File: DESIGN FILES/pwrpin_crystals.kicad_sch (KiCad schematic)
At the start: 34 parts, among them U1 MIMXRT1064CVL5B, Y1 7V24000026, Y2 X201232768KJD2SI

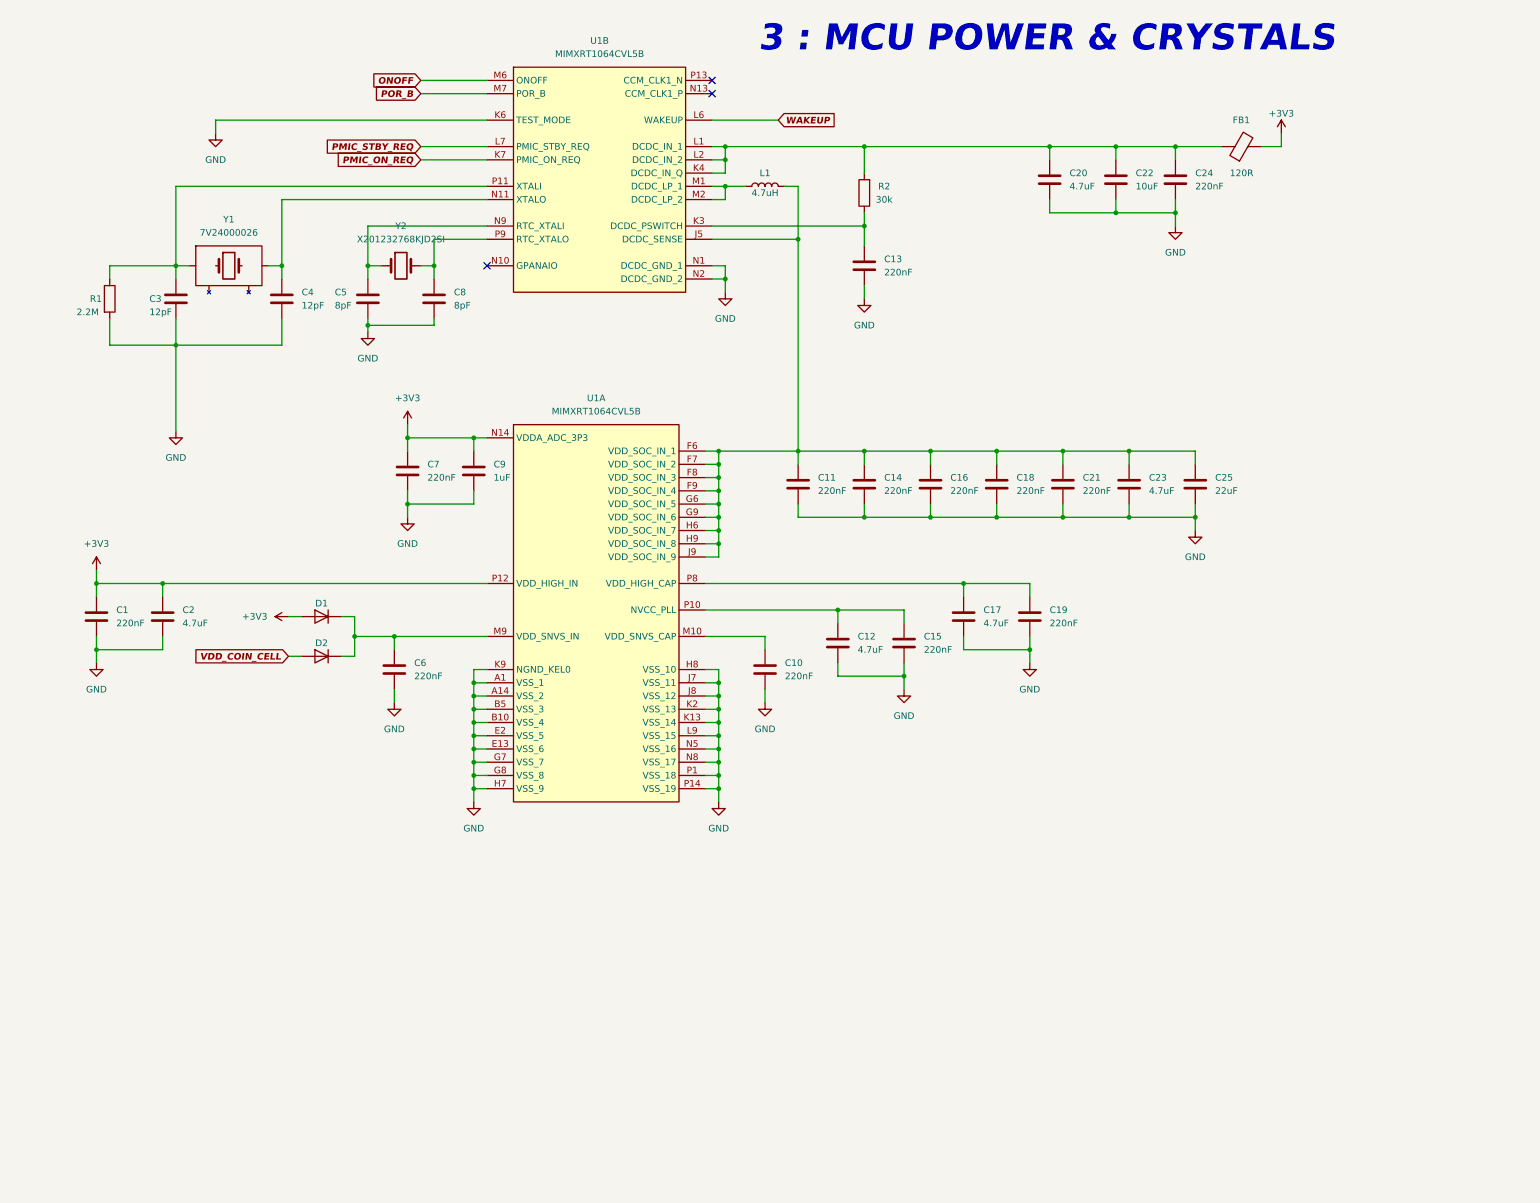
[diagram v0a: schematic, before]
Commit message: schematic edit
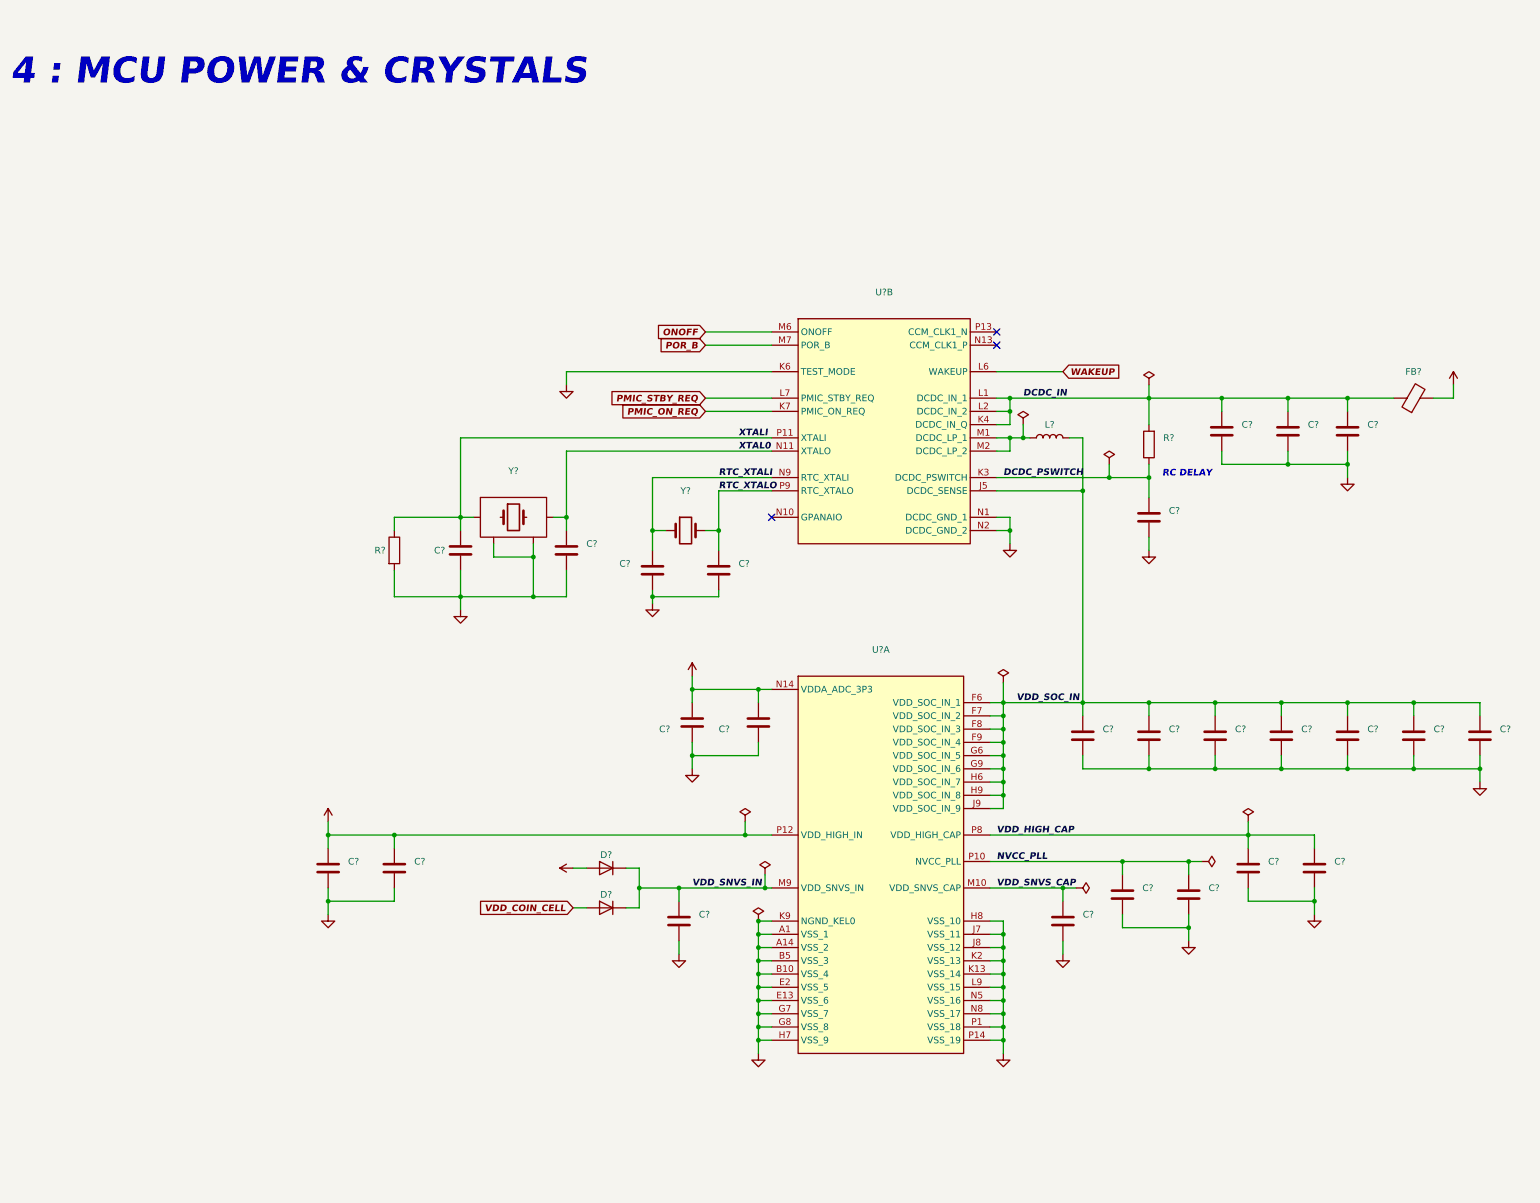
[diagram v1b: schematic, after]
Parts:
- removed C1, C10, C11, C13, C14, C15, C16, C18, C19, C21, C24, C6, C7: 220nF, MIMXRT1064 MCU Module:0402_CL05B224KO5NNNC, symbol MIMXRT1064 MCU Module:CL05B224KO5NNNC
- removed C12, C17, C2, C20, C23: 4.7uF, MIMXRT1064 MCU Module:0402_CL05A475MP5NRNC, symbol MIMXRT1064 MCU Module:CL05A475MP5NRNC
- removed C22: 10uF, MIMXRT1064 MCU Module:0603_CL10A106KP8NNNC, symbol MIMXRT1064 MCU Module:CL10A106KP8NNNC
- removed C25: 22uF, MIMXRT1064 MCU Module:0603_CL10A226MQ8NRNC, symbol MIMXRT1064 MCU Module:CL10A226MQ8NRNC
- removed C3, C4: 12pF, MIMXRT1064 MCU Module:0402_GRM1555C1H120GA01D, symbol MIMXRT1064 MCU Module:GRM1555C1H120GA01D
- removed C5, C8: 8pF, MIMXRT1064 MCU Module:0402_GCM1555C1H8R0DA16D, symbol MIMXRT1064 MCU Module:GCM1555C1H8R0DA16D
- removed C9: 1uF, MIMXRT1064 MCU Module:0402_CL05A105KA5NQNC, symbol MIMXRT1064 MCU Module:CL05A105KA5NQNC
- removed D1, D2: RB521S30_R1_00001, MIMXRT1064 MCU Module:RB521S30_R1_00001, symbol MIMXRT1064 MCU Module:RB521S30_R1_00001
- removed FB1: 120R, MIMXRT1064 MCU Module:0603_BLM18AG121SN1D, symbol MIMXRT1064 MCU Module:BLM18AG121SN1D
- removed L1: 4.7uH, MIMXRT1064 MCU Module:CD32YP0302-4R7M, symbol MIMXRT1064 MCU Module:CD32YP0302-4R7M
- removed R1: 2.2M, MIMXRT1064 MCU Module:0402WGJ0225TCE, symbol MIMXRT1064 MCU Module:0402WGJ0225TCE
- removed R2: 30k, MIMXRT1064 MCU Module:TC0225F3002TCE, symbol MIMXRT1064 MCU Module:TC0225F3002TCE
- removed U1: MIMXRT1064CVL5B, MIMXRT1064 MCU Module:MIMXRT1064CVL5B, symbol MIMXRT1064 MCU Module:MIMXRT1064CVL5B
- removed Y1: 7V24000026, MIMXRT1064 MCU Module:7V24000026, symbol MIMXRT1064 MCU Module:7V24000026
- removed Y2: X201232768KJD2SI, MIMXRT1064 MCU Module:X201232768KJD2SI, symbol MIMXRT1064 MCU Module:X201232768KJD2SI
- added C? (x13): ~, symbol MIMXRT1064 MCU Module:CL05B224KO5NNNC
- added C?: ~, symbol MIMXRT1064 MCU Module:CL10A106KP8NNNC
- added C? (x2): ~, symbol MIMXRT1064 MCU Module:GCM1555C1H8R0DA16D
- added C?: ~, symbol MIMXRT1064 MCU Module:CL05A105KA5NQNC
- added C? (x5): ~, symbol MIMXRT1064 MCU Module:CL05A475MP5NRNC
- added C?: ~, symbol MIMXRT1064 MCU Module:CL10A226MQ8NRNC
- added C? (x2): ~, symbol MIMXRT1064 MCU Module:GRM1555C1H120GA01D
- added D? (x2): ~, symbol MIMXRT1064 MCU Module:RB521S30_R1_00001
- added FB?: ~, symbol MIMXRT1064 MCU Module:BLM18AG121SN1D
- added L?: ~, symbol MIMXRT1064 MCU Module:CD32YP0302-4R7M
- added R?: ~, symbol MIMXRT1064 MCU Module:TC0225F3002TCE
- added R?: ~, symbol MIMXRT1064 MCU Module:0402WGJ0225TCE
- added U? (x2): ~, symbol MIMXRT1064 MCU Module:MIMXRT1064CVL5B
- added Y?: ~, symbol MIMXRT1064 MCU Module:X201232768KJD2SI
- added Y?: ~, symbol MIMXRT1064 MCU Module:7V24000026
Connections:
- net +3V3: now also C?.1, C?.1, C?.1, C?.1, FB?.2, U?.N14 (VDDA_ADC_3P3), U?.P12 (VDD_HIGH_IN)
- net GND: now also C?.2, C?.2, C?.2, C?.2, C?.2, C?.2, C?.2, C?.2, C?.2, C?.2, C?.2, C?.2, C?.2, C?.2, C?.2, C?.2, C?.2, C?.2, C?.2, C?.2, C?.2, C?.2, C?.2, C?.2, C?.2, R?.2, U?.A1 (VSS_1), U?.A14 (VSS_2), U?.B10 (VSS_4), U?.B5 (VSS_3), U?.E13 (VSS_6), U?.E2 (VSS_5), U?.G7 (VSS_7), U?.G8 (VSS_8), U?.H7 (VSS_9), U?.H8 (VSS_10), U?.J7 (VSS_11), U?.J8 (VSS_12), U?.K13 (VSS_14), U?.K2 (VSS_13), U?.K6 (TEST_MODE), U?.K9 (NGND_KEL0), U?.L9 (VSS_15), U?.N1 (DCDC_GND_1), U?.N2 (DCDC_GND_2), U?.N5 (VSS_16), U?.N8 (VSS_17), U?.P1 (VSS_18), U?.P14 (VSS_19), Y?.2 (GND), Y?.4 (GND)
- net ONOFF: now also U?.M6 (ONOFF)
- net PMIC_ON_REQ: now also U?.K7 (PMIC_ON_REQ)
- net PMIC_STBY_REQ: now also U?.L7 (PMIC_STBY_REQ)
- net POR_B: now also U?.M7 (POR_B)
- net VDD_COIN_CELL: now also D?.2 (A)
- net WAKEUP: now also U?.L6 (WAKEUP)
- new net: L?.1, U?.M1 (DCDC_LP_1), U?.M2 (DCDC_LP_2)
- new net DCDC_IN: C?.1, C?.1, C?.1, FB?.1, R?.2, U?.K4 (DCDC_IN_Q), U?.L1 (DCDC_IN_1), U?.L2 (DCDC_IN_2)
- new net DCDC_PSWITCH: C?.1, R?.1, U?.K3 (DCDC_PSWITCH)
- new net NVCC_PLL: C?.1, C?.1, U?.P10 (NVCC_PLL)
- new net RTC_XTALI: C?.1, U?.N9 (RTC_XTALI), Y?.1
- new net RTC_XTALO: C?.1, U?.P9 (RTC_XTALO), Y?.2
- new net VDD_HIGH_CAP: C?.1, C?.1, U?.P8 (VDD_HIGH_CAP)
- new net VDD_SNVS_3V3: D?.2 (A)
- new net VDD_SNVS_CAP: C?.1, U?.M10 (VDD_SNVS_CAP)
- new net VDD_SNVS_IN: C?.1, D?.1 (K), D?.1 (K), U?.M9 (VDD_SNVS_IN)
- new net VDD_SOC_IN: C?.1, C?.1, C?.1, C?.1, C?.1, C?.1, C?.1, L?.2, U?.F6 (VDD_SOC_IN_1), U?.F7 (VDD_SOC_IN_2), U?.F8 (VDD_SOC_IN_3), U?.F9 (VDD_SOC_IN_4), U?.G6 (VDD_SOC_IN_5), U?.G9 (VDD_SOC_IN_6), U?.H6 (VDD_SOC_IN_7), U?.H9 (VDD_SOC_IN_8), U?.J5 (DCDC_SENSE), U?.J9 (VDD_SOC_IN_9)
- new net XTAL0: C?.1, U?.N11 (XTALO), Y?.3
- new net XTALI: C?.1, R?.1, U?.P11 (XTALI), Y?.1
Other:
- note added: "4 : MCU POWER & CRYSTALS"
- note added: "RC DELAY"
- note removed: "3 : MCU POWER & CRYSTALS"
- title: MCU Power & Crystals -> MCU GPIO & Memory signals

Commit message: schematic changes
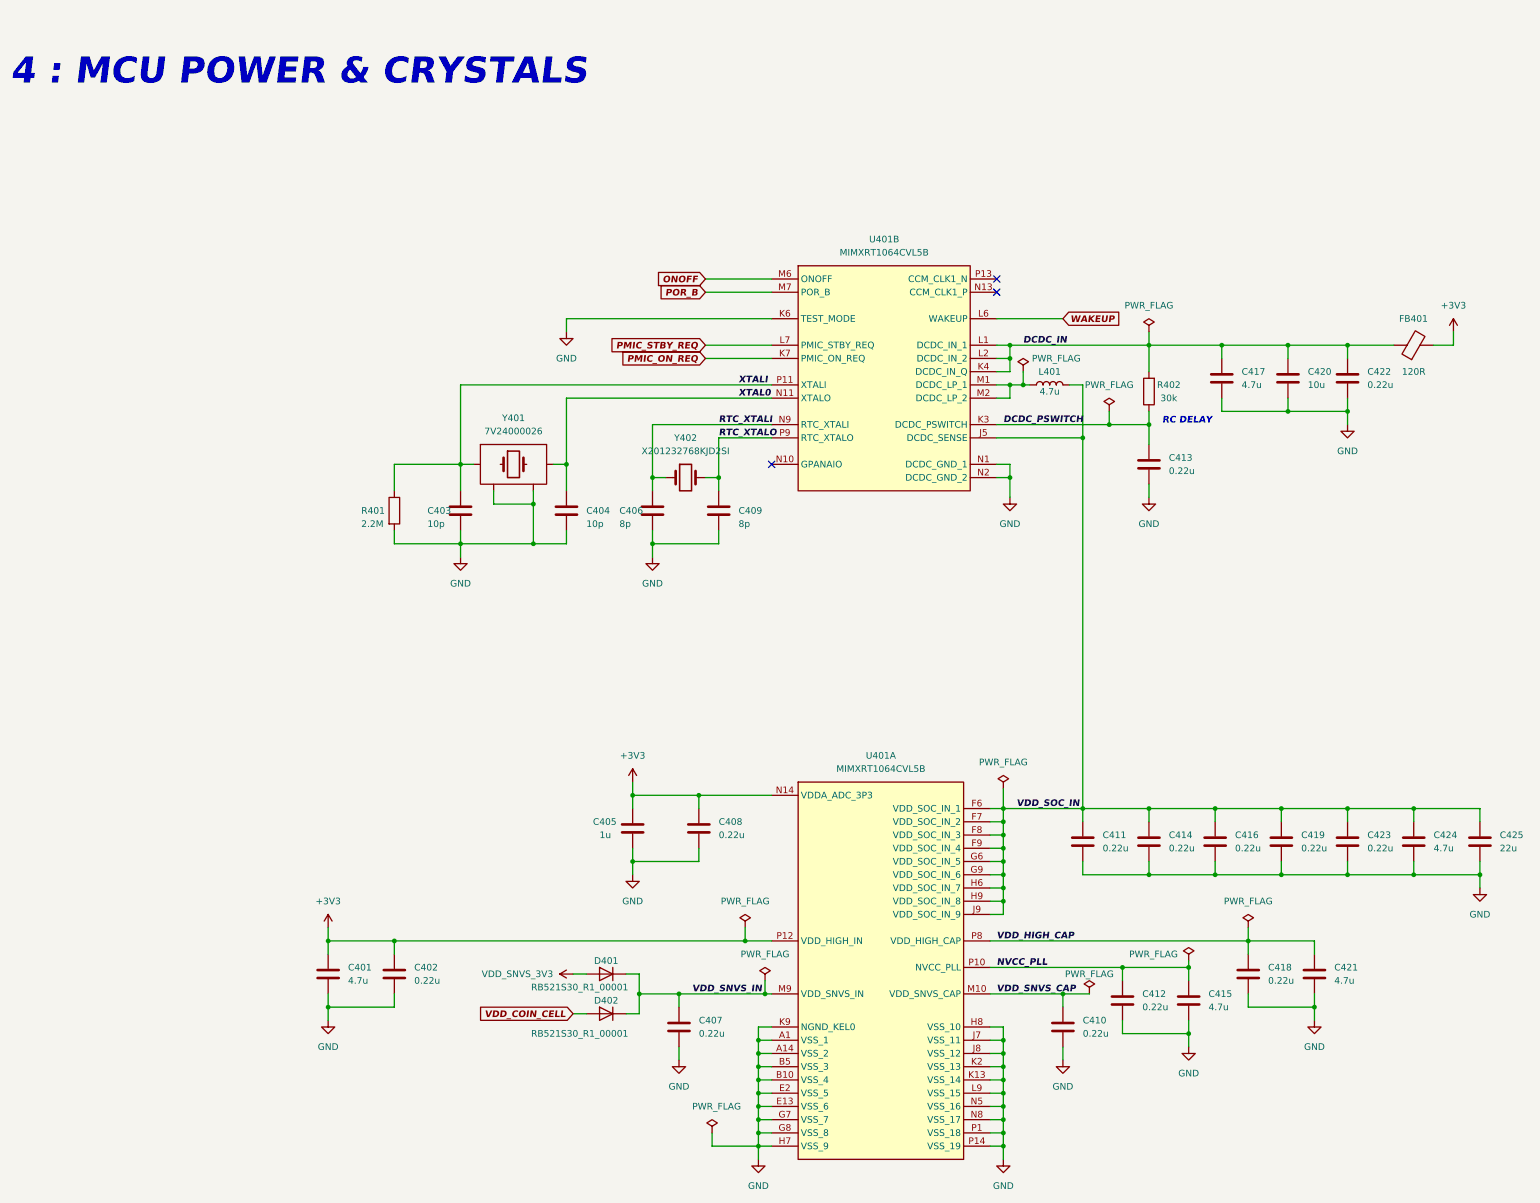
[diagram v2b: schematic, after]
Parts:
- C401, C415, C417, C421, C424: renamed from C?; value ~ -> 4.7u
- C402, C407, C408, C410, C411, C412, C413, C414, C416, C418, C419, C422, C423: renamed from C?; value ~ -> 0.22u
- C403, C404: renamed from C?; value ~ -> 10p
- C405: renamed from C?; value ~ -> 1u
- C406, C409: renamed from C?; value ~ -> 8p
- C420: renamed from C?; value ~ -> 10u
- C425: renamed from C?; value ~ -> 22u
- D401, D402: renamed from D?; value ~ -> RB521S30_R1_00001
- FB401: renamed from FB?; value ~ -> 120R
- L401: renamed from L?; value ~ -> 4.7u
- R401: renamed from R?; value ~ -> 2.2M
- R402: renamed from R?; value ~ -> 30k
- U401: renamed from U?; value ~ -> MIMXRT1064CVL5B
- Y401: renamed from Y?; value ~ -> 7V24000026
- Y402: renamed from Y?; value ~ -> X201232768KJD2SI
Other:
- moved on the sheet: C401, C402, C403, C404, C405, C406, C407, C408, C409, C410, C411, C412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
